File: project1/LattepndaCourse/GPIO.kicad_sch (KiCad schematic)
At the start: 0 parts

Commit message: Hierachi
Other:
- title: (none) -> practice design
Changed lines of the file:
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@@
 	(generator "eeschema")
 	(generator_version "9.0")
-	(paper "A4")
+	(paper "A2")
+	(title_block
+		(title "practice design")
+		(date "2026-09-30")
+		(rev "1")
+	)
 )

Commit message: working on GPIO
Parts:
- added J4, J5, J6, J7: Conn_01x04_Pin, A_HDJ_Library:PinHeader_1x03_P2.54mm_Vertical, symbol Connector:Conn_01x04_Pin
- added U5, U6, U7, U8, U9: ULC0524P, A_HDJ_Library:Diodes_UDFN-10_1.0x2.5mm_P0.5mm, symbol Power_Protection:D3V3XA4B10LP
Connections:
- new net: U6.3 (VSS), U6.8 (VSS)
- new net: U9.3 (VSS), U9.8 (VSS)
- new net: U8.3 (VSS), U8.8 (VSS)
- new net +3V3: J7.1 (Pin_1), J7.2 (Pin_2), J7.3 (Pin_3), J7.4 (Pin_4)
- new net GND: J6.1 (Pin_1), J6.2 (Pin_2), J6.3 (Pin_3), J6.4 (Pin_4), U5.3 (VSS), U5.8 (VSS), U7.3 (VSS), U7.8 (VSS)
- new net I2C2_SCL: J5.1 (Pin_1), U7.1, U7.10 (NC)
- new net I2C2_SDA: J4.1 (Pin_1), U5.1, U5.10 (NC)
- new net I2C3_SCL: J5.2 (Pin_2), U7.2, U7.9 (NC)
- new net I2C3_SDA: J4.2 (Pin_2), U5.2, U5.9 (NC)
- new net I2C4_SCL: J5.3 (Pin_3), U7.4, U7.7 (NC)
- new net I2C4_SDA: J4.3 (Pin_3), U5.4, U5.7 (NC)
- new net I2C5_SCL: J5.4 (Pin_4), U7.5, U7.6 (NC)
- new net I2C5_SDA: J4.4 (Pin_4), U5.5, U5.6 (NC)

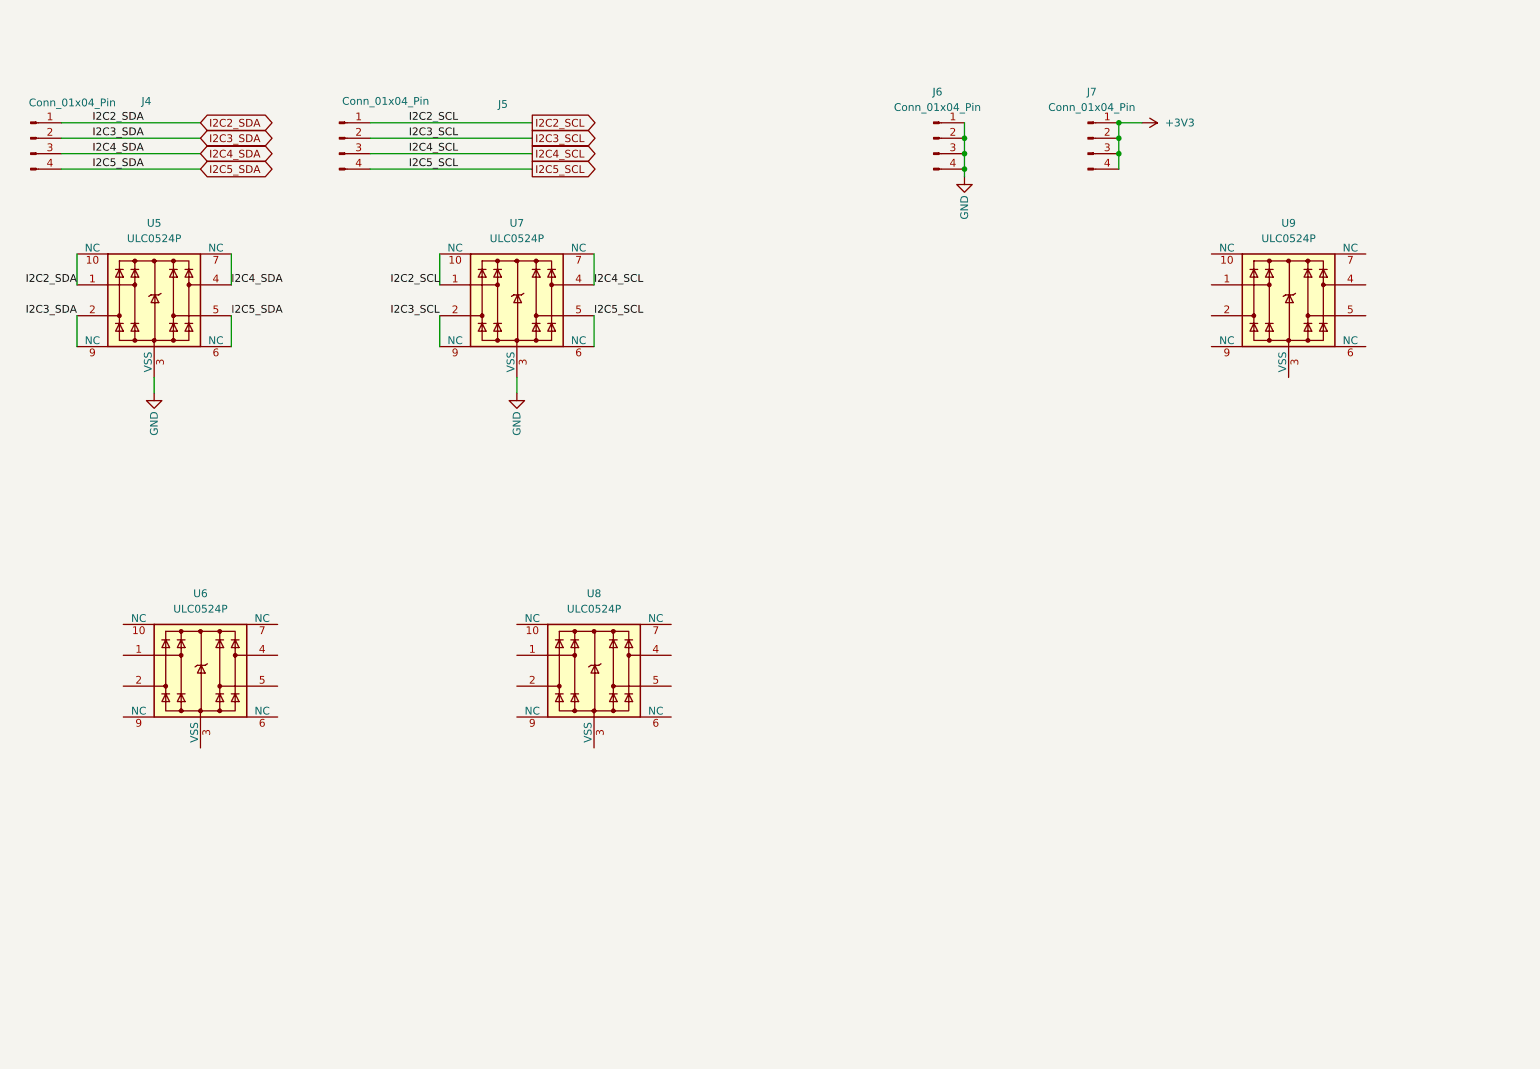
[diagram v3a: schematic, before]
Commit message: GPIO is done
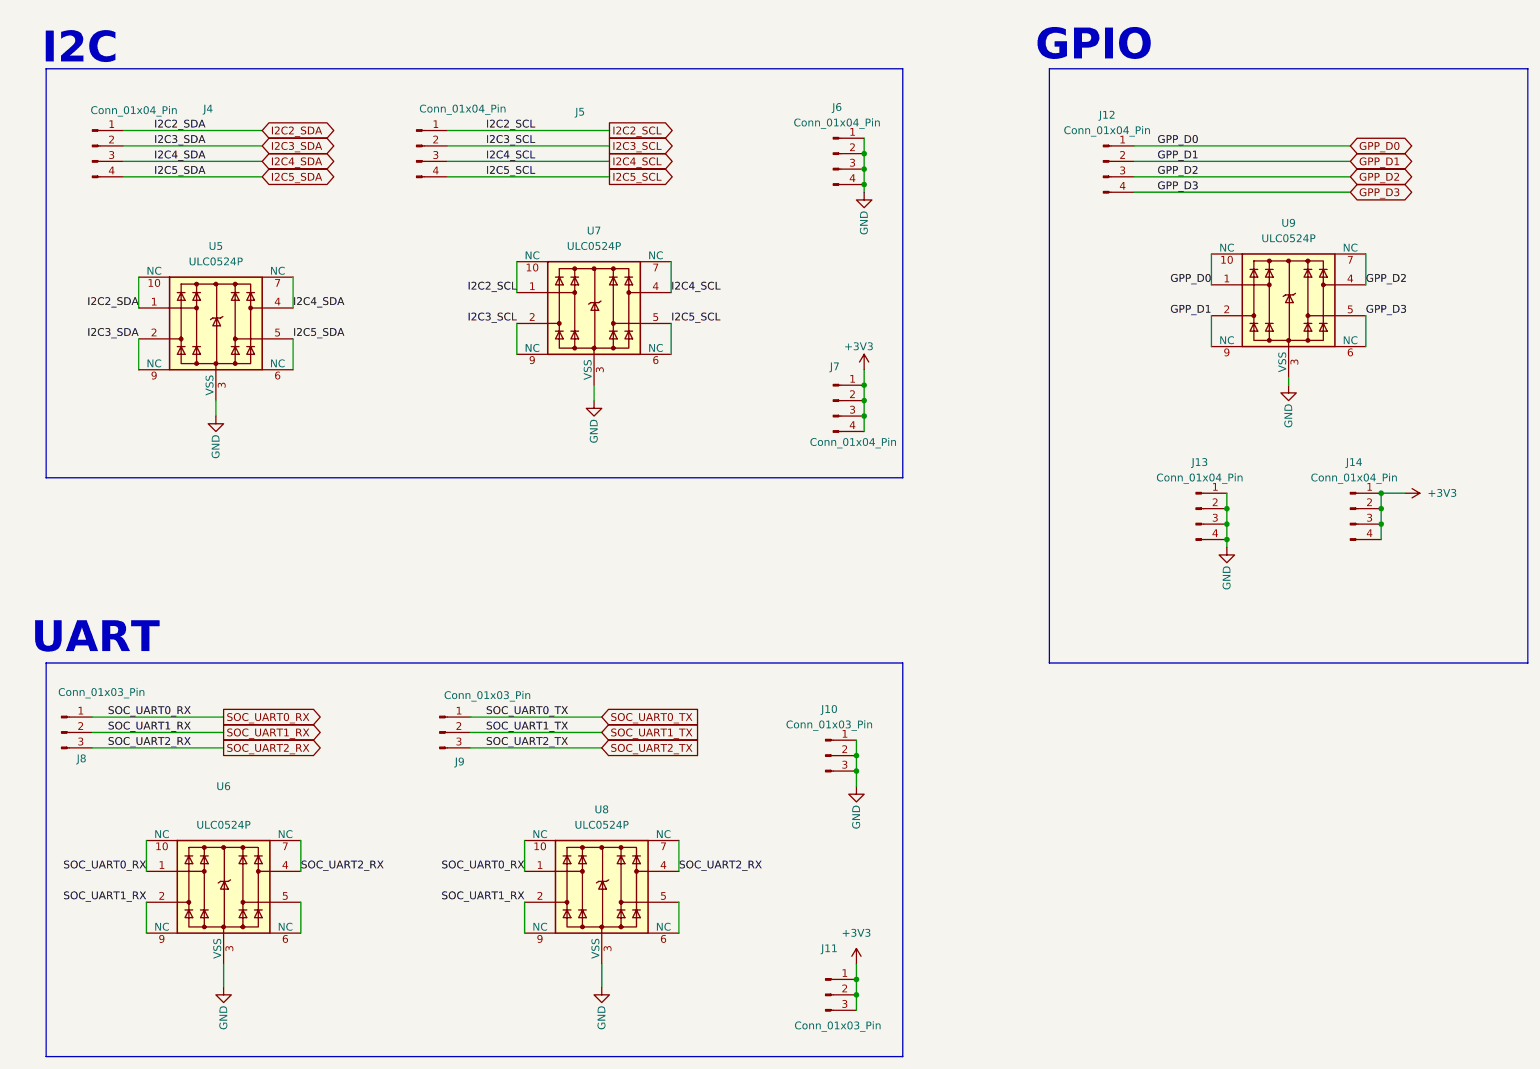
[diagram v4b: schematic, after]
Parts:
- added J10, J11, J8, J9: Conn_01x03_Pin, A_HDJ_Library:PinHeader_1x03_P2.54mm_Vertical, symbol Connector:Conn_01x03_Pin
- added J12, J13, J14: Conn_01x04_Pin, A_HDJ_Library:PinHeader_1x03_P2.54mm_Vertical, symbol Connector:Conn_01x04_Pin
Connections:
- net +3V3: now also J11.1 (Pin_1), J11.2 (Pin_2), J11.3 (Pin_3), J14.1 (Pin_1), J14.2 (Pin_2), J14.3 (Pin_3), J14.4 (Pin_4)
- net GND: now also U6.3 (VSS), U6.8 (VSS), U8.3 (VSS), U8.8 (VSS), U9.3 (VSS), U9.8 (VSS), J10.1 (Pin_1), J10.2 (Pin_2), J10.3 (Pin_3), J13.1 (Pin_1), J13.2 (Pin_2), J13.3 (Pin_3), J13.4 (Pin_4)
- net SOC_UART0_RX: now reaches U6.1
- net SOC_UART0_RX: now also U6.10 (NC), U8.1, U8.10 (NC), J8.1 (Pin_1)
- net SOC_UART1_RX: now reaches U6.2
- net SOC_UART1_RX: now also U6.9 (NC), U8.2, U8.9 (NC), J8.2 (Pin_2)
- net SOC_UART2_RX: now reaches U6.4
- net SOC_UART2_RX: now also U6.7 (NC), U8.4, U8.7 (NC), J8.3 (Pin_3)
- net at U6.5: now also U6.6 (NC)
- net GPP_D0: now reaches U9.1
- net GPP_D0: now also U9.10 (NC), J12.1 (Pin_1)
- net GPP_D1: now reaches U9.2
- net GPP_D1: now also U9.9 (NC), J12.2 (Pin_2)
- net GPP_D2: now reaches U9.4
- net GPP_D2: now also U9.7 (NC), J12.3 (Pin_3)
- net GPP_D3: now reaches U9.5
- net GPP_D3: now also U9.6 (NC), J12.4 (Pin_4)
- net at U8.5: now also U8.6 (NC)
- new net SOC_UART0_TX: J9.1 (Pin_1)
- new net SOC_UART1_TX: J9.2 (Pin_2)
- new net SOC_UART2_TX: J9.3 (Pin_3)
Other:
- note added: "GPIO"
- note added: "I2C"
- note added: "UART"
- moved on the sheet: J4, J5, J6, J7, U5, U6, U7, U8

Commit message: Hierachi needs some work
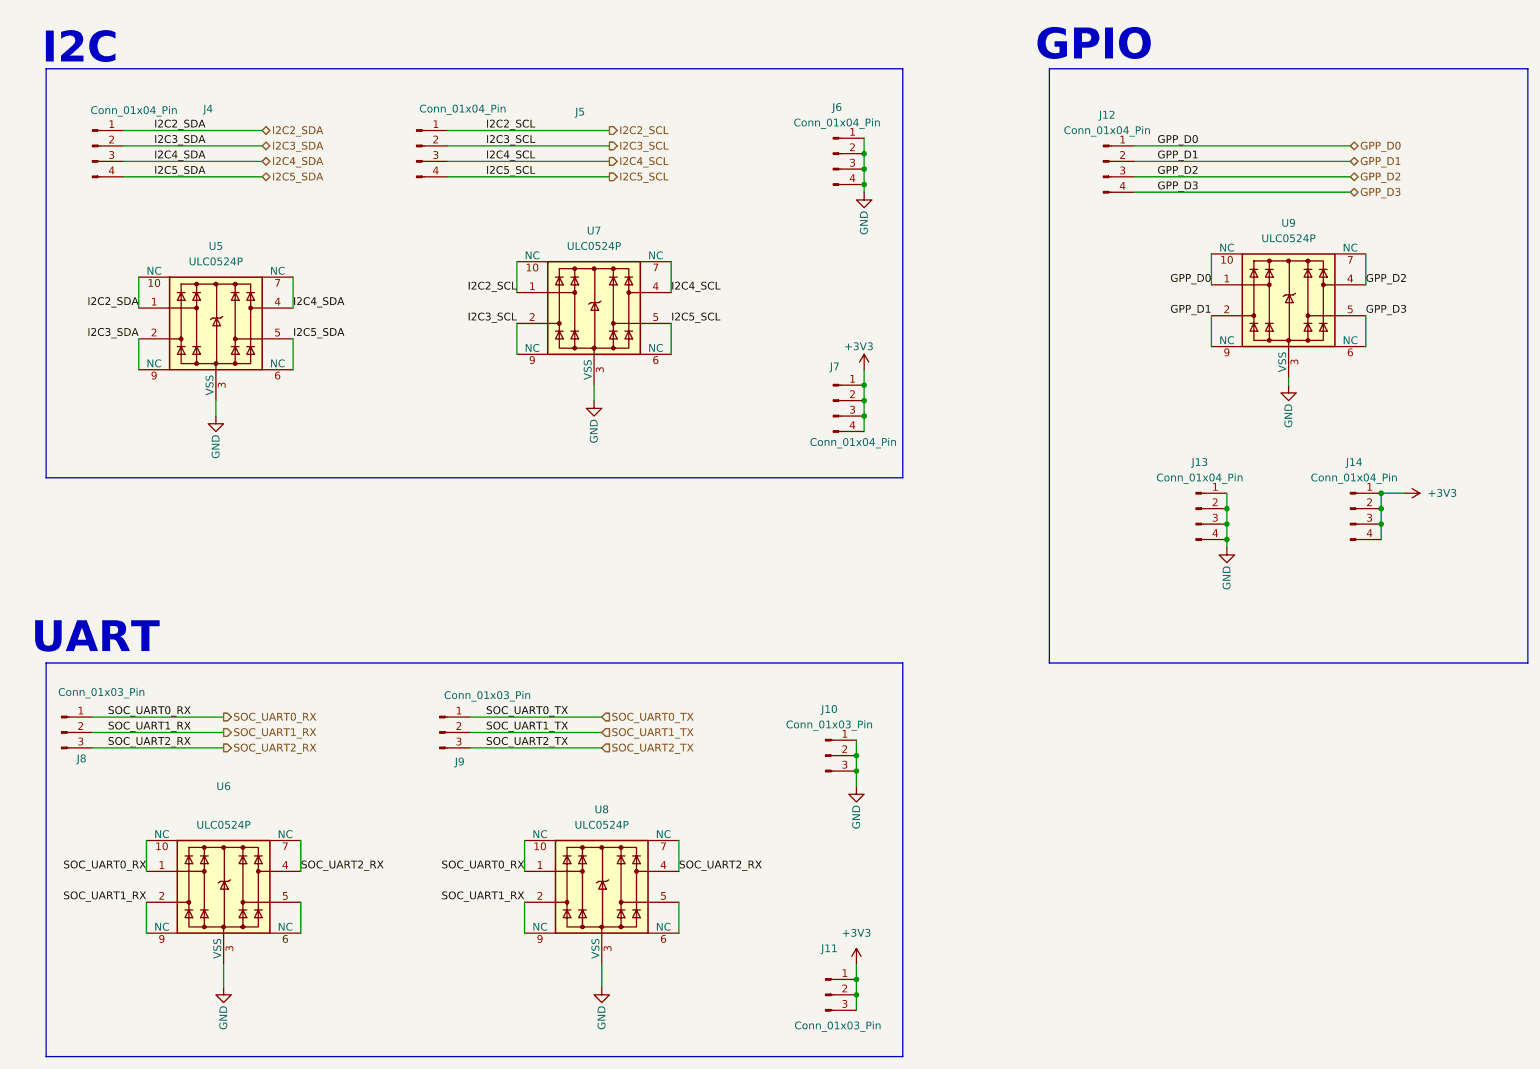
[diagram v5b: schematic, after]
